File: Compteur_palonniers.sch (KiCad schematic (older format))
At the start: 12 parts, among them J1 Conn_01x05, J101 Connecteur_Nextion, J2 Conn_01x04, K101 RelaisSRD, U1 MP1584, U2 ATtiny85

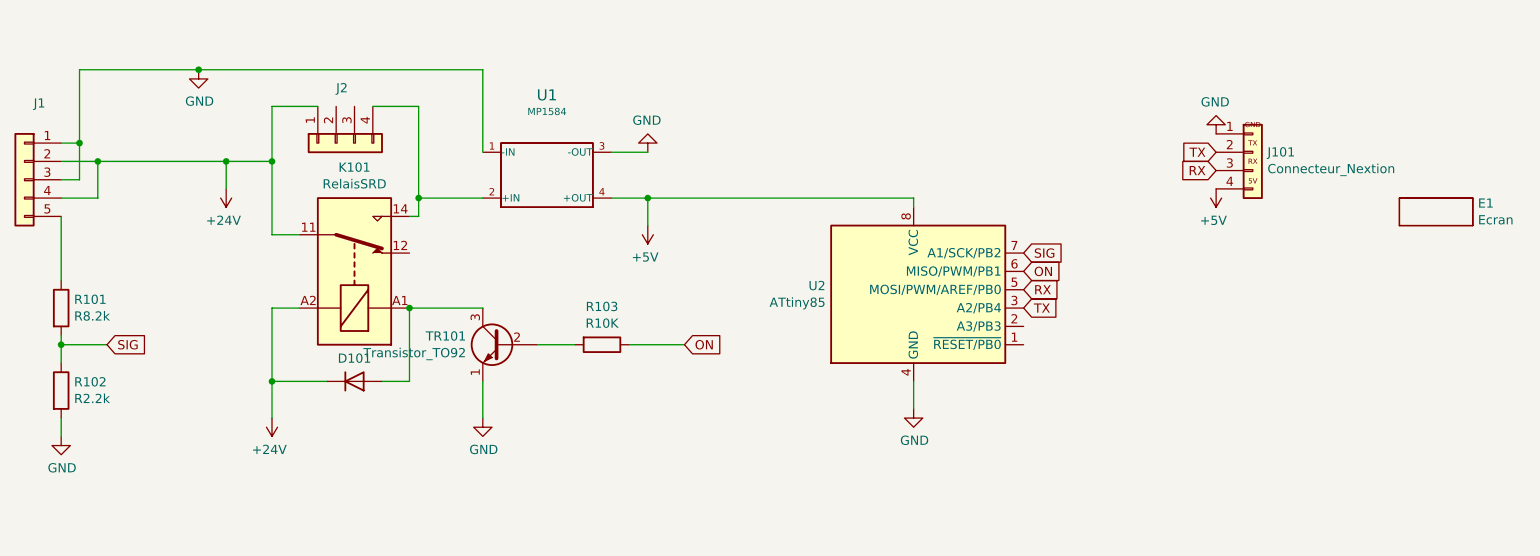
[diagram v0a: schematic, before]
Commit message: Modif alim
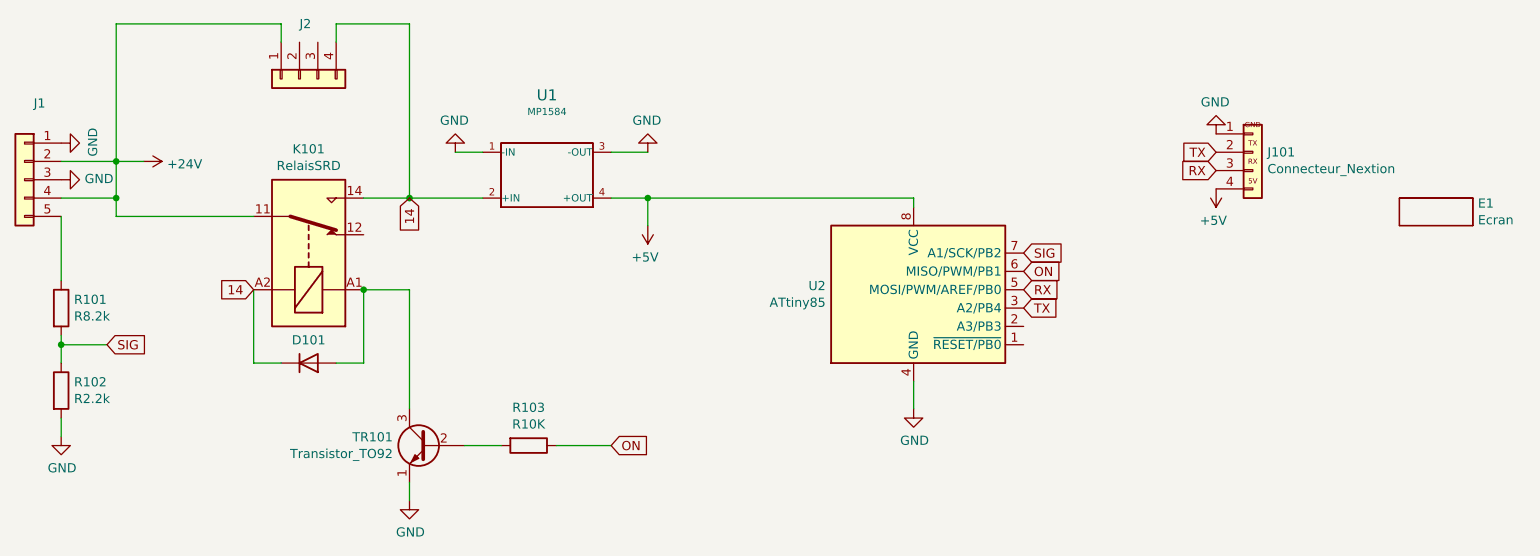
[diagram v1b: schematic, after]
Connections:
- net +24V: no longer D101.1 (K), K101.A2
- net 14: now reaches J2.4 (Pin_4), K101.14, U1.2 (+IN)
- net 14: now also D101.1 (K), K101.A2
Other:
- moved on the sheet: D101, J2, K101, R103, TR101
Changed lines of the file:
@@
 RX
-$Comp
-L power:+24V #PWR0102
-U 1 1 6432E81D
-P 3050 2150
-F 0 "#PWR0102" H 3050 2000 50  0001 C CNN
-F 1 "+24V" H 3065 2323 50  0000 C CNN
-F 2 "" H 3050 2150 50  0001 C CNN
-F 3 "" H 3050 2150 50  0001 C CNN
-	1    3050 2150
-	-1   0    0    1
-$EndComp
 $Comp
 L power:+5V #PWR0103
@@
 Wire Wire Line
 	6800 3350 6800 3200
-Text GLabel 5550 3000 2    50   Input ~ 0
+Text GLabel 5150 3550 2    50   Input ~ 0
 ON
 Text GLabel 7400 2600 2    50   Input ~ 0
@@
 Wire Wire Line
 	2150 2300 2150 2650
-Wire Wire Line
-	3050 2150 3050 2000
 $Comp
 L Personnel:Ecran E1
@@
 $EndComp
 Wire Wire Line
-	2150 2000 2350 2000
-Wire Wire Line
-	2150 1900 2250 1900
-Connection ~ 3050 2000
-Wire Wire Line
-	3050 2000 3300 2000
-Wire Wire Line
-	2150 2100 2250 2100
-Wire Wire Line
-	2250 2100 2250 1900
-Wire Wire Line
-	2150 2200 2350 2200
-Wire Wire Line
-	2350 2200 2350 2000
-Connection ~ 2350 2000
-Wire Wire Line
-	2350 2000 3050 2000
-Wire Wire Line
 	6800 2200 6800 2250
 Connection ~ 5350 2200
@@
 	1    0    0    -1
 $EndComp
-Wire Wire Line
-	3300 1700 3300 2000
-Connection ~ 3300 2000
-Wire Wire Line
-	4100 1700 4100 2200
-Wire Wire Line
-	4100 2200 4450 2200
-Wire Wire Line
-	2250 1900 2250 1500
-Wire Wire Line
-	4450 1500 4450 1950
-Connection ~ 2250 1900
 $Comp
 L Connector_Generic:Conn_01x04 J2
 U 1 1 643D02A0
-P 3650 1900
-F 0 "J2" V 3350 1900 50  0000 R CNN
-F 1 "Conn_01x04" V 3613 1612 50  0001 R CNN
-F 2 "pin_2_54mm:pin_strip_4" H 3650 1900 50  0001 C CNN
-F 3 "~" H 3650 1900 50  0001 C CNN
-	1    3650 1900
+P 3450 1550
+F 0 "J2" V 3150 1550 50  0000 R CNN
+F 1 "Conn_01x04" V 3413 1262 50  0001 R CNN
+F 2 "pin_2_54mm:pin_strip_4" H 3450 1550 50  0001 C CNN
+F 3 "~" H 3450 1550 50  0001 C CNN
+	1    3450 1550
 	0    -1   1    0
 $EndComp
-Wire Wire Line
-	3550 1700 3300 1700
-Wire Wire Line
-	3850 1700 4100 1700
 $Comp
 L Personnel:ATtiny85 U2
@@
 $EndComp
 Wire Wire Line
-	5250 3000 5550 3000
+	4850 3550 5150 3550
 $Comp
 L Personnel:RelaisSRD K101
 U 1 1 6439057C
-P 3750 2600
-F 0 "K101" V 4317 2600 50  0000 C CNN
-F 1 "RelaisSRD" V 4226 2600 50  0000 C CNN
-F 2 "Relay_THT:Relais_SRD" H 5020 2570 50  0001 C CNN
-F 3 "https://gfinder.findernet.com/public/attachments/36/EN/S36EN.pdf" H 3750 2600 50  0001 C CNN
-	1    3750 2600
+P 3500 2500
+F 0 "K101" V 4067 2500 50  0000 C CNN
+F 1 "RelaisSRD" V 3976 2500 50  0000 C CNN
+F 2 "Relay_THT:Relais_SRD" H 4770 2470 50  0001 C CNN
+F 3 "https://gfinder.findernet.com/public/attachments/36/EN/S36EN.pdf" H 3500 2500 50  0001 C CNN
+	1    3500 2500
 	0    1    -1   0
 $EndComp
-Wire Wire Line
-	3450 2400 3300 2400
-Wire Wire Line
-	3300 2000 3300 2400
-Wire Wire Line
-	4050 2300 4100 2300
-Wire Wire Line
-	4100 2300 4100 2200
-Connection ~ 4100 2200
-Wire Wire Line
-	3450 2800 3300 2800
-Wire Wire Line
-	3300 2800 3300 3200
 $Comp
 L Personnel:Diode_1N4148 D101
 U 1 1 6439AB6F
-P 3750 3200
-F 0 "D101" H 3750 3075 50  0000 C CNN
-F 1 "Diode_1N4148" H 3750 3100 50  0001 C CNN
-F 2 "pth_diodes:diode_do35" H 3750 3025 50  0001 C CNN
-F 3 "" H 3750 3200 50  0001 C CNN
-	1    3750 3200
+P 3500 3100
+F 0 "D101" H 3500 2975 50  0000 C CNN
+F 1 "Diode_1N4148" H 3500 3000 50  0001 C CNN
+F 2 "pth_diodes:diode_do35" H 3500 2925 50  0001 C CNN
+F 3 "" H 3500 3100 50  0001 C CNN
+	1    3500 3100
 	1    0    0    1
 $EndComp
-Wire Wire Line
-	3600 3200 3300 3200
-Wire Wire Line
-	3900 3200 4050 3200
-Wire Wire Line
-	4050 3200 4050 2800
 $Comp
 L Personnel:Transistor_TO92 TR101
 U 1 1 6439D8F7
-P 4550 3000
-F 0 "TR101" H 4741 3046 50  0000 L CNN
-F 1 "Transistor_TO92" H 4741 2955 50  0000 L CNN
-F 2 "Transistor:TO-92" H 4750 2925 50  0001 L CIN
-F 3 "" H 4550 3000 50  0001 L CNN
-	1    4550 3000
+P 4150 3550
+F 0 "TR101" H 4341 3596 50  0000 L CNN
+F 1 "Transistor_TO92" H 4341 3505 50  0000 L CNN
+F 2 "Transistor:TO-92" H 4350 3475 50  0001 L CIN
+F 3 "" H 4150 3550 50  0001 L CNN
+	1    4150 3550
 	-1   0    0    -1
 $EndComp
 Wire Wire Line
 	2150 3400 2150 3500
-Wire Wire Line
-	4050 2800 4450 2800
-Connection ~ 4050 2800
 $Comp
 L power:GND #PWR0106
 U 1 1 643A273A
-P 4450 3400
-F 0 "#PWR0106" H 4450 3150 50  0001 C CNN
-F 1 "GND" H 4455 3227 50  0000 C CNN
-F 2 "" H 4450 3400 50  0001 C CNN
-F 3 "" H 4450 3400 50  0001 C CNN
-	1    4450 3400
-	1    0    0    -1
-$EndComp
-Wire Wire Line
-	3300 3400 3300 3200
-Connection ~ 3300 3200
-Wire Wire Line
-	4450 3400 4450 3200
+P 4050 3850
+F 0 "#PWR0106" H 4050 3600 50  0001 C CNN
+F 1 "GND" H 4055 3677 50  0000 C CNN
+F 2 "" H 4050 3850 50  0001 C CNN
+F 3 "" H 4050 3850 50  0001 C CNN
+	1    4050 3850
+	1    0    0    -1
+$EndComp
 $Comp
 L Personnel:R R103
 U 1 1 643A4D4E
-P 5100 3000
-F 0 "R103" V 4893 3000 50  0000 C CNN
-F 1 "R10K" V 4984 3000 50  0000 C CNN
-F 2 "Resistance:R_025W" V 5030 3000 50  0001 C CNN
-F 3 "~" H 5100 3000 50  0001 C CNN
-	1    5100 3000
+P 4700 3550
+F 0 "R103" V 4493 3550 50  0000 C CNN
+F 1 "R10K" V 4584 3550 50  0000 C CNN
+F 2 "Resistance:R_025W" V 4630 3550 50  0001 C CNN
+F 3 "~" H 4700 3550 50  0001 C CNN
+	1    4700 3550
 	0    1    1    0
 $EndComp
 Wire Wire Line
-	4950 3000 4750 3000
+	4550 3550 4350 3550
 $Comp
 L Personnel:Connecteur_Nextion J101
@@
 Wire Wire Line
 	5350 2200 6800 2200
-Wire Wire Line
-	2250 1500 2900 1500
 $Comp
 L power:GND #PWR0108
 U 1 1 643A447E
-P 2900 1500
-F 0 "#PWR0108" H 2900 1250 50  0001 C CNN
-F 1 "GND" H 2905 1327 50  0000 C CNN
-F 2 "" H 2900 1500 50  0001 C CNN
-F 3 "" H 2900 1500 50  0001 C CNN
-	1    2900 1500
-	1    0    0    -1
-$EndComp
-Connection ~ 2900 1500
-Wire Wire Line
-	2900 1500 4450 1500
+P 2150 1900
+F 0 "#PWR0108" H 2150 1650 50  0001 C CNN
+F 1 "GND" H 2155 1727 50  0000 C CNN
+F 2 "" H 2150 1900 50  0001 C CNN
+F 3 "" H 2150 1900 50  0001 C CNN
+	1    2150 1900
+	0    -1   -1   0
+$EndComp
 $Comp
 L power:GND #PWR0101
@@
 Wire Wire Line
 	5150 1950 5350 1950
+Wire Wire Line
+	3800 2200 4050 2200
+$Comp
+L power:GND #PWR0102
+U 1 1 6465AB97
+P 2150 2100
+F 0 "#PWR0102" H 2150 1850 50  0001 C CNN
+F 1 "GND" V 2155 1972 50  0000 R CNN
+F 2 "" H 2150 2100 50  0001 C CNN
+F 3 "" H 2150 2100 50  0001 C CNN
+	1    2150 2100
+	0    -1   -1   0
+$EndComp
 $Comp
 L power:+24V #PWR0107
-U 1 1 643A7B46
-P 3300 3400
-F 0 "#PWR0107" H 3300 3250 50  0001 C CNN
-F 1 "+24V" H 3315 3573 50  0000 C CNN
-F 2 "" H 3300 3400 50  0001 C CNN
-F 3 "" H 3300 3400 50  0001 C CNN
-	1    3300 3400
-	-1   0    0    1
-$EndComp
+U 1 1 6465C036
+P 2600 2000
+F 0 "#PWR0107" H 2600 1850 50  0001 C CNN
+F 1 "+24V" V 2615 2128 50  0000 L CNN
+F 2 "" H 2600 2000 50  0001 C CNN
+F 3 "" H 2600 2000 50  0001 C CNN
+	1    2600 2000
+	0    1    1    0
+$EndComp
+Wire Wire Line
+	2450 2200 2150 2200
+Wire Wire Line
+	2150 2000 2450 2000
+Wire Wire Line
+	2450 2200 2450 2000
+Connection ~ 2450 2000
+Wire Wire Line
+	2450 2000 2600 2000
+Wire Wire Line
+	3350 1350 3350 1250
+Wire Wire Line
+	3350 1250 2450 1250
+Wire Wire Line
+	2450 1250 2450 2000
+Wire Wire Line
+	3200 2300 2450 2300
+Wire Wire Line
+	2450 2300 2450 2200
+Connection ~ 2450 2200
+Wire Wire Line
+	3650 1350 3650 1250
+Wire Wire Line
+	3650 1250 4050 1250
+Wire Wire Line
+	4050 1250 4050 2200
+Connection ~ 4050 2200
+Wire Wire Line
+	4050 2200 4450 2200
+Wire Wire Line
+	3800 2700 4050 2700
+Wire Wire Line
+	4050 3850 4050 3750
+$Comp
+L power:GND #PWR0109
+U 1 1 64670522
+P 4300 1950
+F 0 "#PWR0109" H 4300 1700 50  0001 C CNN
+F 1 "GND" H 4305 1777 50  0000 C CNN
+F 2 "" H 4300 1950 50  0001 C CNN
+F 3 "" H 4300 1950 50  0001 C CNN
+	1    4300 1950
+	-1   0    0    1
+$EndComp
+Wire Wire Line
+	4300 1950 4450 1950
+Wire Wire Line
+	4050 2700 4050 3350
+Wire Wire Line
+	3200 2700 3200 3100
+Wire Wire Line
+	3200 3100 3350 3100
+Wire Wire Line
+	3650 3100 3800 3100
+Wire Wire Line
+	3800 3100 3800 2700
+Connection ~ 3800 2700
+Text GLabel 4050 2200 3    50   Input ~ 0
+14
+Text GLabel 3200 2700 0    50   Input ~ 0
+14
 $EndSCHEMATC
